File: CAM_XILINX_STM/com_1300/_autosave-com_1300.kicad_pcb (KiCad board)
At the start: 4 copper layers, 50 x 75.9 mm, 104 parts, among them IC1 XC3S400-4TQ144C, IC2 SN74CBTD3384CDBR, IC3 SN74CBTD3384CDBR, IC4 SN74CBTD3384CDBR, IC5 SN74CBTD3384CDBR, J1 Conn_02x04_Top_Bottom, J2 Conn_02x04_Top_Bottom, J3 Conn_02x03_Top_Bottom, J4 9-68RD-0.635SF, U1 LT1963AxST-3.3, U2 LP3982IMM-ADJ, U3 LTC3411EMS, U4 STM32F415RGTx, U5 AM29LV320DT90EC, U6 TC74LCX373FT, Y1 40mHZ, Y2 16mHz

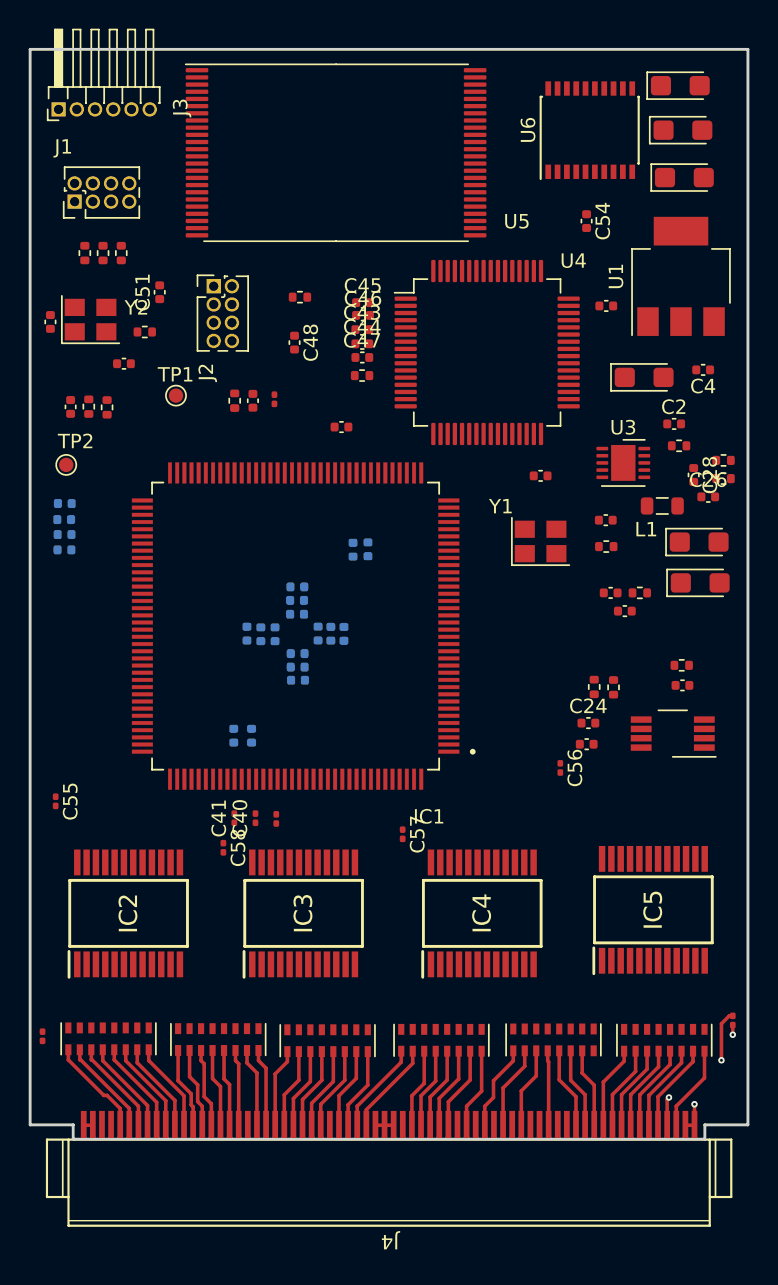
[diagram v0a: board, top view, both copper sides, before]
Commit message: 453254\
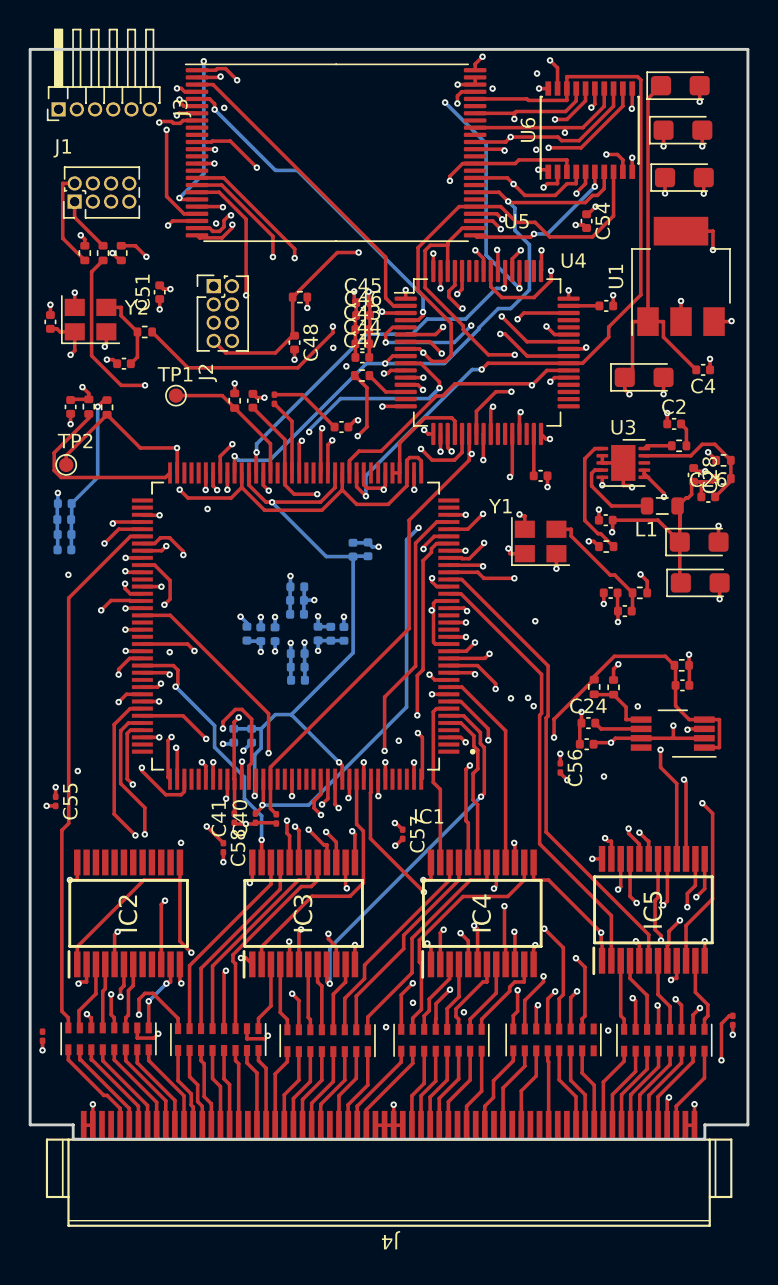
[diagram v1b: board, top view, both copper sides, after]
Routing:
- net GND: track 11.3 -> 133.0 mm, vias 2 -> 82
- net +2V5: track 0.00 -> 119.1 mm, vias 0 -> 5
- net BUS_OE: track 0.00 -> 111.1 mm, vias 0 -> 7
- net VCC: track 1.27 -> 106.4 mm, vias 0 -> 6
- net uC_CNTRL2: track 0.00 -> 91.2 mm, vias 0 -> 5
- net +1V2: track 0.00 -> 90.7 mm, vias 0 -> 4
- net uC_CNTRL4: track 0.00 -> 76.1 mm, vias 0 -> 4
- net INOUT_MDO3: track 0.00 -> 66.3 mm, vias 0 -> 3
- net INOUT_MDO4: track 0.00 -> 63.8 mm, vias 0 -> 3
- net _D2: track 0.00 -> 63.8 mm, vias 0 -> 3
- net uC_CNTRL1: track 0.00 -> 63.7 mm, vias 0 -> 2
- net uC_CNTRL3: track 0.00 -> 60.9 mm, vias 0 -> 3
- net _D0: track 0.00 -> 60.4 mm, vias 0 -> 3
- net _D1: track 0.00 -> 59.5 mm, vias 0 -> 3
- net INOUT_MDO5: track 0.00 -> 58.8 mm, vias 0 -> 3
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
